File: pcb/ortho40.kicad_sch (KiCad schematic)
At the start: 129 parts, among them J1 SWD, J2 USB_C_Receptacle_USB2.0, SW1 SW_Push, U1 RP2040, U2 XC6206PxxxMR, U3 W25Q128JVS, U4 USBLC6-2SC6, U5 ST7735S_1.8inch, Y1 12MHz

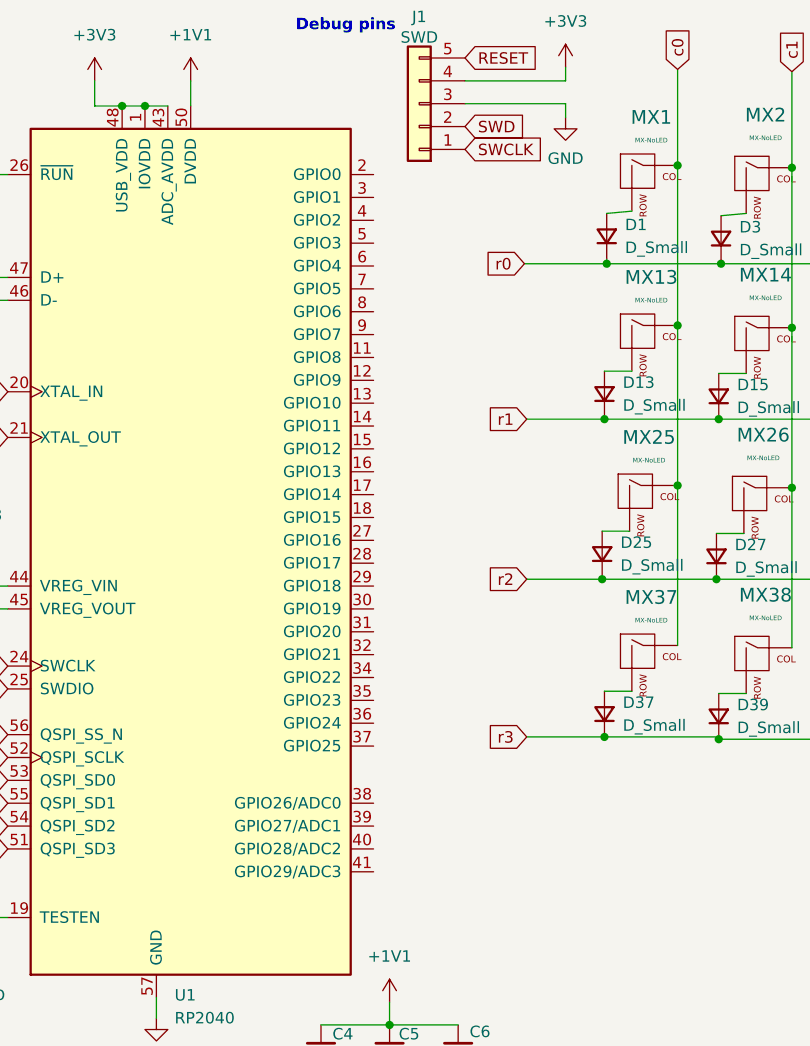
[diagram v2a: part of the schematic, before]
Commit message: Fully finish PCB
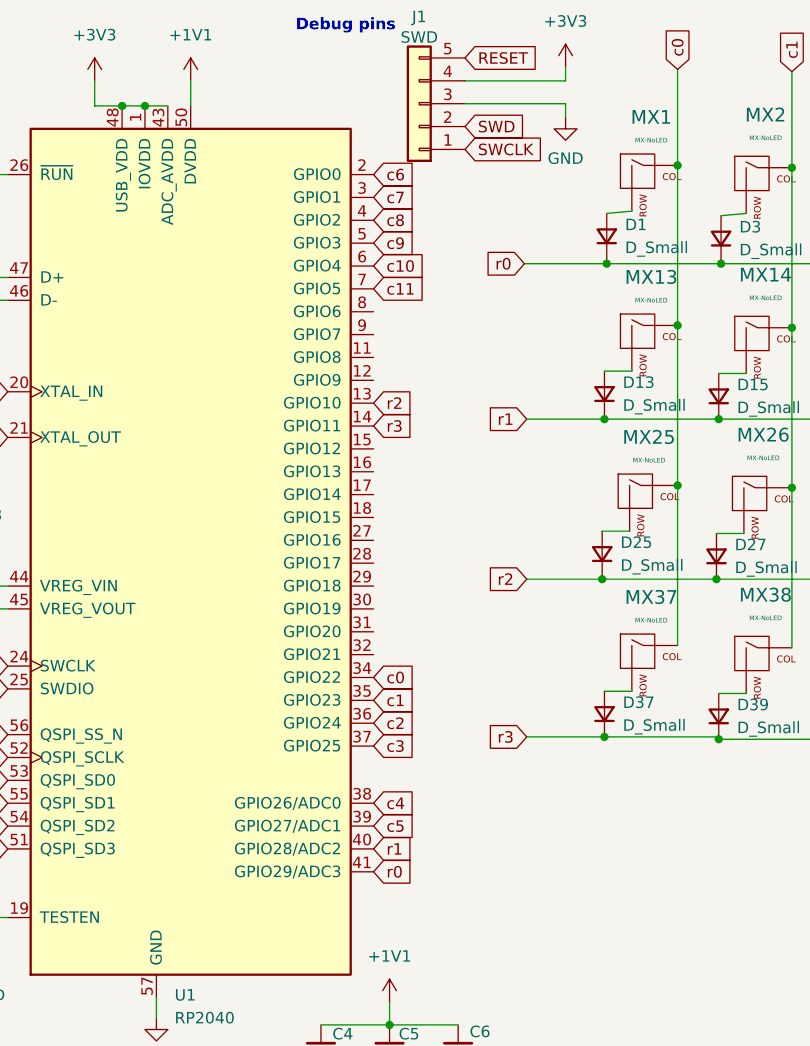
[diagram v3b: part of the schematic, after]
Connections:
- net c0: now also U1.34 (GPIO22)
- net c1: now also U1.35 (GPIO23)
- net c10: now also U1.6 (GPIO4)
- net c11: now also U1.7 (GPIO5)
- net c2: now also U1.36 (GPIO24)
- net c3: now also U1.37 (GPIO25)
- net c4: now also U1.38 (GPIO26/ADC0)
- net c5: now also U1.39 (GPIO27/ADC1)
- net c6: now also U1.2 (GPIO0)
- net c7: now also U1.3 (GPIO1)
- net c8: now also U1.4 (GPIO2)
- net c9: now also U1.5 (GPIO3)
- net r0: now also U1.41 (GPIO29/ADC3)
- net r1: now also U1.40 (GPIO28/ADC2)
- net r2: now also U1.13 (GPIO10)
- net r3: now also U1.14 (GPIO11)
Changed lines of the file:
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@@
     (effects (font (size 1.27 1.27) italic) (justify left bottom))
   )
+  (global_label "c4" (shape input) (at 76.708 100.584 0) (fields_autoplaced)
+    (effects (font (size 1.27 1.27)) (justify left))
+    (property "Intersheet References" "${INTERSHEET_REFS}" (id 0) (at 81.4192 100.5046 0)
+      (effects (font (size 1.27 1.27)) (justify left) hide)
+    )
+  )
   (global_label "LCD_RESET" (shape input) (at 43.942 168.91 180) (fields_autoplaced)
     (effects (font (size 1.27 1.27)) (justify right))
@@
     )
   )
+  (global_label "c11" (shape input) (at 76.708 43.434 0) (fields_autoplaced)
+    (effects (font (size 1.27 1.27)) (justify left))
+    (property "Intersheet References" "${INTERSHEET_REFS}" (id 0) (at 82.6287 43.3546 0)
+      (effects (font (size 1.27 1.27)) (justify left) hide)
+    )
+  )
   (global_label "USB_DP" (shape input) (at 258.826 131.572 0) (fields_autoplaced)
     (effects (font (size 1.27 1.27)) (justify left))
@@
     )
   )
+  (global_label "c2" (shape input) (at 76.708 91.694 0) (fields_autoplaced)
+    (effects (font (size 1.27 1.27)) (justify left))
+    (property "Intersheet References" "${INTERSHEET_REFS}" (id 0) (at 81.4192 91.6146 0)
+      (effects (font (size 1.27 1.27)) (justify left) hide)
+    )
+  )
   (global_label "SWCLK" (shape input) (at 86.868 27.94 0) (fields_autoplaced)
     (effects (font (size 1.27 1.27)) (justify left))
@@
     )
   )
+  (global_label "r2" (shape input) (at 76.708 56.134 0) (fields_autoplaced)
+    (effects (font (size 1.27 1.27)) (justify left))
+    (property "Intersheet References" "${INTERSHEET_REFS}" (id 0) (at 81.1168 56.0546 0)
+      (effects (font (size 1.27 1.27)) (justify left) hide)
+    )
+  )
   (global_label "DN" (shape input) (at 220.98 148.336 0) (fields_autoplaced)
     (effects (font (size 1.27 1.27)) (justify left))
@@
     )
   )
+  (global_label "c7" (shape input) (at 76.708 33.274 0) (fields_autoplaced)
+    (effects (font (size 1.27 1.27)) (justify left))
+    (property "Intersheet References" "${INTERSHEET_REFS}" (id 0) (at 81.4192 33.1946 0)
+      (effects (font (size 1.27 1.27)) (justify left) hide)
+    )
+  )
   (global_label "CLK_OUT" (shape input) (at 178.816 152.908 0) (fields_autoplaced)
     (effects (font (size 1.27 1.27)) (justify left))
@@
     )
   )
+  (global_label "c6" (shape input) (at 76.708 30.734 0) (fields_autoplaced)
+    (effects (font (size 1.27 1.27)) (justify left))
+    (property "Intersheet References" "${INTERSHEET_REFS}" (id 0) (at 81.4192 30.6546 0)
+      (effects (font (size 1.27 1.27)) (justify left) hide)
+    )
+  )
   (global_label "c9" (shape input) (at 224.79 19.558 90) (fields_autoplaced)
     (effects (font (size 1.27 1.27)) (justify left))
@@
     )
   )
+  (global_label "r1" (shape input) (at 76.708 105.664 0) (fields_autoplaced)
+    (effects (font (size 1.27 1.27)) (justify left))
+    (property "Intersheet References" "${INTERSHEET_REFS}" (id 0) (at 81.1168 105.5846 0)
+      (effects (font (size 1.27 1.27)) (justify left) hide)
+    )
+  )
   (global_label "LCD_DC" (shape input) (at 43.942 171.45 180) (fields_autoplaced)
     (effects (font (size 1.27 1.27)) (justify right))
@@
     )
   )
+  (global_label "c0" (shape input) (at 76.708 86.614 0) (fields_autoplaced)
+    (effects (font (size 1.27 1.27)) (justify left))
+    (property "Intersheet References" "${INTERSHEET_REFS}" (id 0) (at 81.4192 86.5346 0)
+      (effects (font (size 1.27 1.27)) (justify left) hide)
+    )
+  )
   (global_label "QSPI_SD2" (shape input) (at 179.578 128.524 0) (fields_autoplaced)
     (effects (font (size 1.27 1.27)) (justify left))
@@
     )
   )
+  (global_label "c1" (shape input) (at 76.708 89.154 0) (fields_autoplaced)
+    (effects (font (size 1.27 1.27)) (justify left))
+    (property "Intersheet References" "${INTERSHEET_REFS}" (id 0) (at 81.4192 89.0746 0)
+      (effects (font (size 1.27 1.27)) (justify left) hide)
+    )
+  )
   (global_label "CLK_IN" (shape input) (at 178.816 147.828 0) (fields_autoplaced)
     (effects (font (size 1.27 1.27)) (justify left))
@@
     )
   )
+  (global_label "c8" (shape input) (at 76.708 35.814 0) (fields_autoplaced)
+    (effects (font (size 1.27 1.27)) (justify left))
+    (property "Intersheet References" "${INTERSHEET_REFS}" (id 0) (at 81.4192 35.7346 0)
+      (effects (font (size 1.27 1.27)) (justify left) hide)
+    )
+  )
   (global_label "c4" (shape input) (at 161.29 19.304 90) (fields_autoplaced)
     (effects (font (size 1.27 1.27)) (justify left))
@@
     )
   )
+  (global_label "r3" (shape input) (at 76.708 58.674 0) (fields_autoplaced)
+    (effects (font (size 1.27 1.27)) (justify left))
+    (property "Intersheet References" "${INTERSHEET_REFS}" (id 0) (at 81.1168 58.5946 0)
+      (effects (font (size 1.27 1.27)) (justify left) hide)
+    )
+  )
   (global_label "QSPI_SCLK" (shape input) (at 154.178 128.524 180) (fields_autoplaced)
     (effects (font (size 1.27 1.27)) (justify right))
@@
     )
   )
+  (global_label "c3" (shape input) (at 76.708 94.234 0) (fields_autoplaced)
+    (effects (font (size 1.27 1.27)) (justify left))
+    (property "Intersheet References" "${INTERSHEET_REFS}" (id 0) (at 81.4192 94.1546 0)
+      (effects (font (size 1.27 1.27)) (justify left) hide)
+    )
+  )
   (global_label "r1" (shape input) (at 93.726 57.912 180) (fields_autoplaced)
     (effects (font (size 1.27 1.27)) (justify right))
@@
     )
   )
+  (global_label "r0" (shape input) (at 76.708 108.204 0) (fields_autoplaced)
+    (effects (font (size 1.27 1.27)) (justify left))
+    (property "Intersheet References" "${INTERSHEET_REFS}" (id 0) (at 81.1168 108.1246 0)
+      (effects (font (size 1.27 1.27)) (justify left) hide)
+    )
+  )
   (global_label "QSPI_SD0" (shape input) (at 36.068 98.044 180) (fields_autoplaced)
     (effects (font (size 1.27 1.27)) (justify right))
@@
     )
   )
+  (global_label "c5" (shape input) (at 76.708 103.124 0) (fields_autoplaced)
+    (effects (font (size 1.27 1.27)) (justify left))
+    (property "Intersheet References" "${INTERSHEET_REFS}" (id 0) (at 81.4192 103.0446 0)
+      (effects (font (size 1.27 1.27)) (justify left) hide)
+    )
+  )
   (global_label "SWCLK" (shape input) (at 36.068 85.344 180) (fields_autoplaced)
     (effects (font (size 1.27 1.27)) (justify right))
@@
     )
   )
+  (global_label "c9" (shape input) (at 76.708 38.354 0) (fields_autoplaced)
+    (effects (font (size 1.27 1.27)) (justify left))
+    (property "Intersheet References" "${INTERSHEET_REFS}" (id 0) (at 81.4192 38.2746 0)
+      (effects (font (size 1.27 1.27)) (justify left) hide)
+    )
+  )
   (global_label "c1" (shape input) (at 123.19 19.304 90) (fields_autoplaced)
     (effects (font (size 1.27 1.27)) (justify left))
@@
     (property "Intersheet References" "${INTERSHEET_REFS}" (id 0) (at 34.816 161.2106 0)
       (effects (font (size 1.27 1.27)) (justify right) hide)
+    )
+  )
+  (global_label "c10" (shape input) (at 76.708 40.894 0) (fields_autoplaced)
+    (effects (font (size 1.27 1.27)) (justify left))
+    (property "Intersheet References" "${INTERSHEET_REFS}" (id 0) (at 82.6287 40.8146 0)
+      (effects (font (size 1.27 1.27)) (justify left) hide)
     )
   )
@@
     )
     (pin "1")
+    (pin "10")
     (pin "2")
     (pin "3")
@@
     (pin "8")
     (pin "9")
-    (pin "10")
   )
   (symbol (lib_id "Device:R_Small") (at 149.098 123.444 90) (unit 1)
